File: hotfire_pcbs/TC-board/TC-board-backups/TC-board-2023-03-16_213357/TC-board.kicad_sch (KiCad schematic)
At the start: 13 parts, among them J1 DB15_Female, J3 PCIE-LP-01-01-F-DV-A-TR, U1 MAX31856_Breakout, U2 MAX31856_Breakout

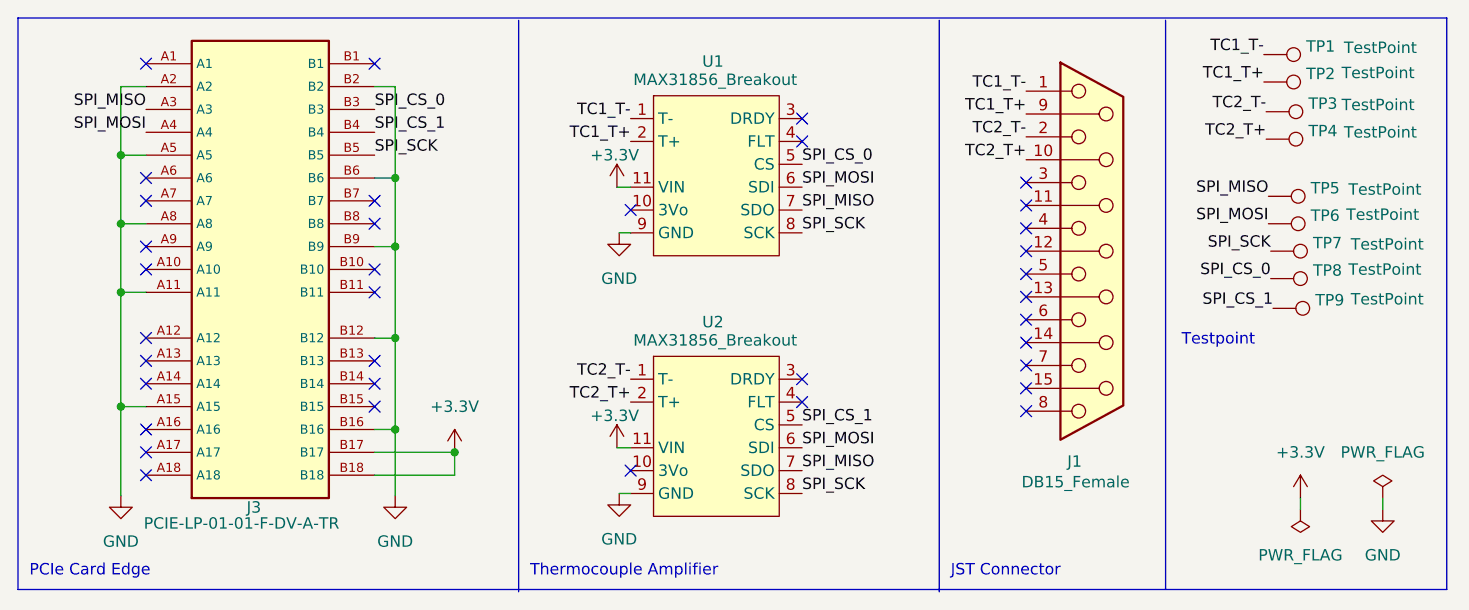
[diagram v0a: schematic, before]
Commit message: Updated TC Board
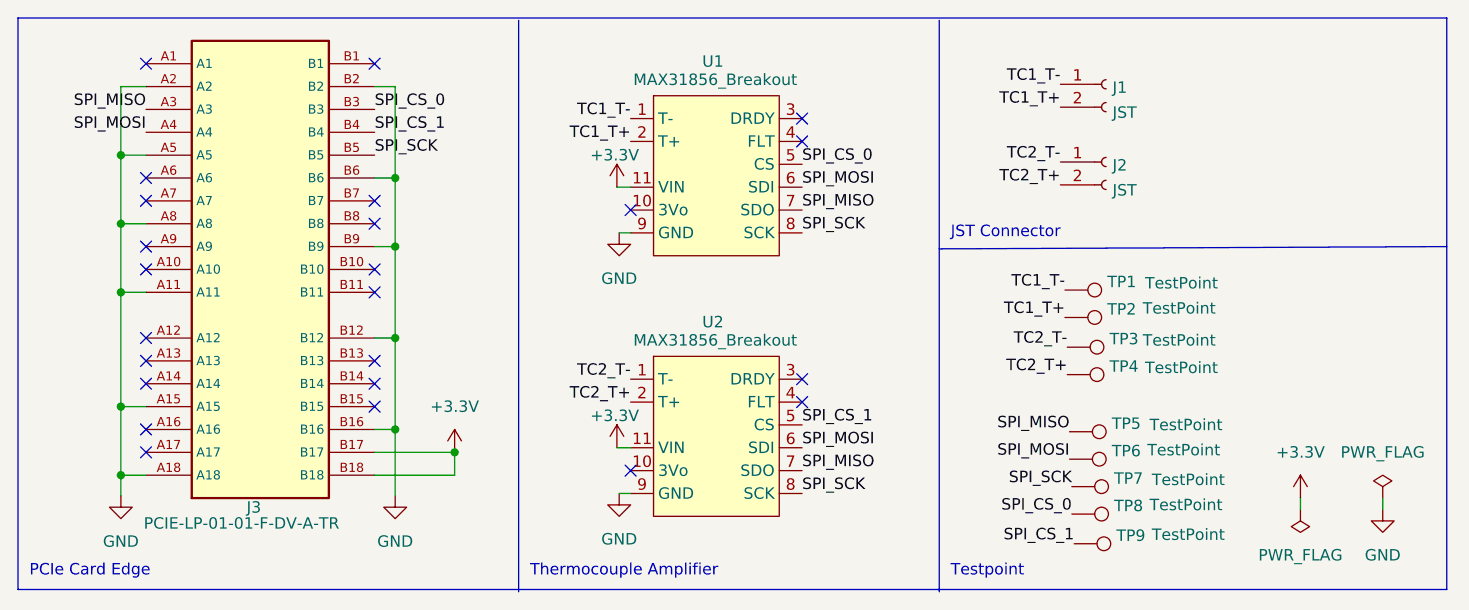
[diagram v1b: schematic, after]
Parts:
- removed J1: DB15_Female, DSUB_622-015-260-042:DSUB_622-015-260-042, symbol Connector:DB15_Female
- added J1, J2: JST, Connector_PinHeader_2.54mm:PinHeader_1x02_P2.54mm_Horizontal, symbol Connector:Conn_01x02_Female
- TP1, TP2, TP3, TP4, TP5, TP6, TP7, TP8, TP9: footprint TestPoint:TestPoint_Keystone_5010-5014_Multipurpose -> TestPoint:TestPoint_Plated_Hole_D2.0mm
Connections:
- net GND: now also J3.A18
- net TC1_T+: now also J1.2 (Pin_2)
- net TC1_T-: now also J1.1 (Pin_1)
- net TC2_T+: now also J2.2 (Pin_2)
- net TC2_T-: now also J2.1 (Pin_1)
- net +3.3V renamed +3V3
- no-connect marks 36 -> 24
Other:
- moved on the sheet: TP1, TP2, TP3, TP4, TP5, TP6, TP7, TP8, TP9
